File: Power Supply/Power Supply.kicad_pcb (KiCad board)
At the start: 2 copper layers, 127 x 101.6 mm, 37 parts, among them J1 Conn_01x01_Female, J2 Conn_01x01_Female, J3 Conn_01x01_Female, J4 -V_Conn, J5 +V_Conn, J6 GND_Conn, U1 LM337_TO220, U2 LM317_3PinPackage

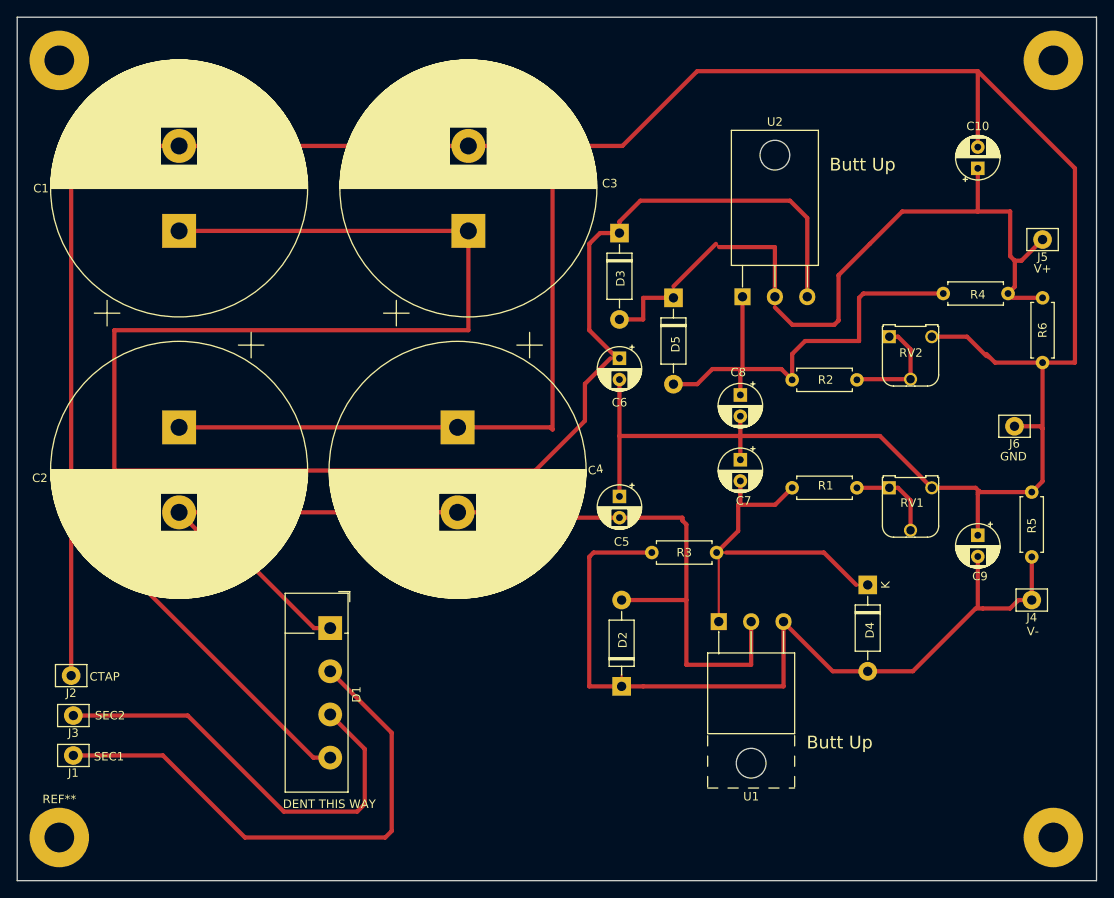
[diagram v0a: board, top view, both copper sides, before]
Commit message: ooh some new pcbs yayy
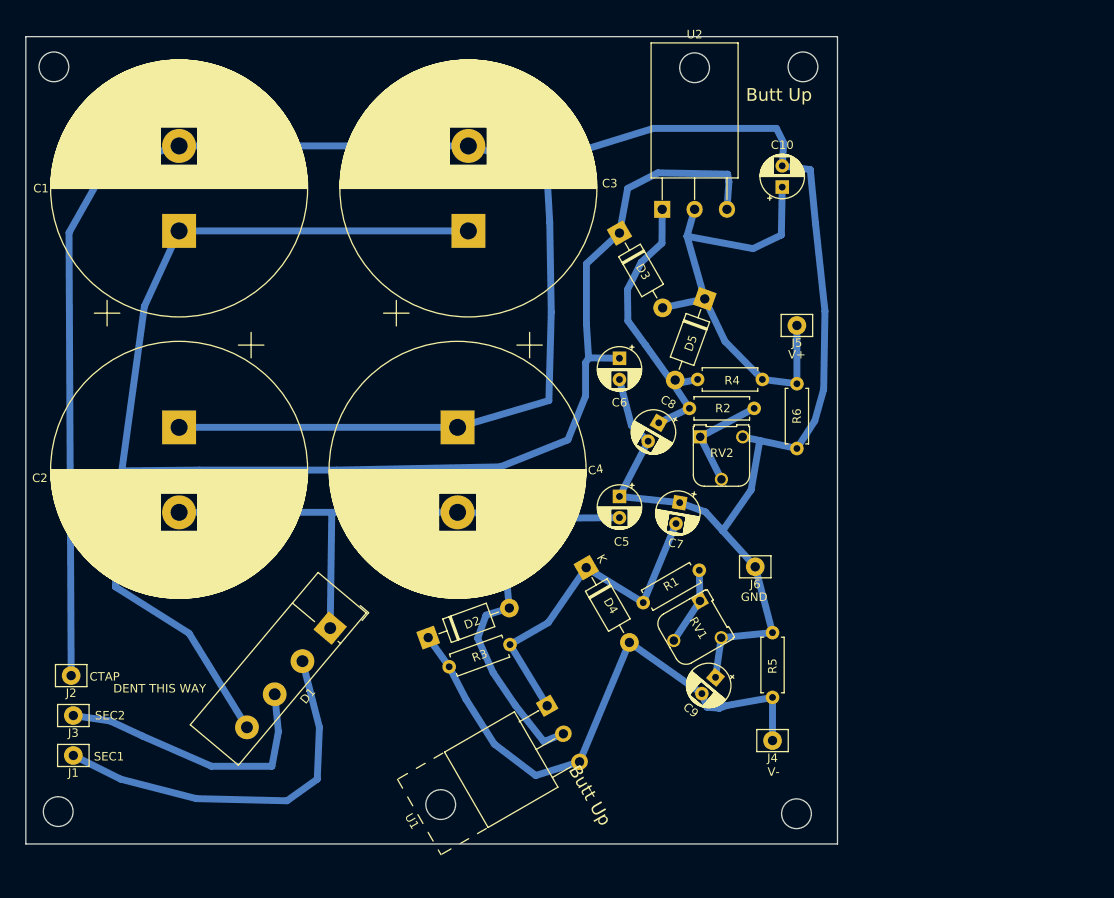
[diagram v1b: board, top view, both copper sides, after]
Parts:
- removed the REF** at (134.6, 17.8)
- removed the REF** at (134.6, 109.2)
- removed the REF** at (17.7, 109.2)
- removed the REF** at (17.7, 17.8)
- added REF**: MountingHole_3.5mm, MountingHole:MountingHole_3.5mm, F.Cu at (17.0, 18.5)
- added REF**: MountingHole_3.5mm, MountingHole:MountingHole_3.5mm, F.Cu at (17.5, 106.2)
- added REF**: MountingHole_3.5mm, MountingHole:MountingHole_3.5mm, F.Cu at (104.4, 106.4)
- added REF**: MountingHole_3.5mm, MountingHole:MountingHole_3.5mm, F.Cu at (105.2, 18.5)
- moved C9 35.1 mm to (94.9, 90.4), turned to 230 degrees
- moved J4 34.7 mm to (101.6, 97.8)
- moved J6 34.7 mm to (99.5, 77.4)
- moved R5 34.7 mm to (101.6, 92.7)
- moved D4 33.2 mm to (79.7, 77.5), turned to 300 degrees
- moved R4 30.6 mm to (100.4, 55.3)
- moved J5 30.6 mm to (104.4, 49.0)
- moved R6 30.6 mm to (104.4, 55.8)
- moved R3 27.4 mm to (63.5, 89.1), turned to 20 degrees
- moved RV1 25.9 mm to (93.0, 81.4), turned to 300 degrees
- moved RV2 25.2 mm to (93.1, 62.1)
- moved U1 23.6 mm to (75.7, 94.8), turned to 300 degrees
- moved D2 23.5 mm to (61.1, 85.7), turned to 20 degrees
- moved C10 23.1 mm to (102.7, 32.7)
- moved R1 22.1 mm to (86.4, 81.6), turned to 30 degrees
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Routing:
- net Earth: track 412.0 -> 327.1 mm
- net Net-(C1-Pad1): track 271.2 -> 205.5 mm
- net Net-(C10-Pad1): track 93.5 -> 56.7 mm
- net /VNEG: track 101.4 -> 66.6 mm
- net Net-(C2-Pad2): track 120.8 -> 99.4 mm
- net Net-(C8-Pad1): track 54.0 -> 34.1 mm
- net /SEC1: track 63.6 -> 44.6 mm
- net Net-(D1-Pad3): track 51.6 -> 33.1 mm
- net Net-(C7-Pad2): track 45.5 -> 39.4 mm
- net Net-(R1-Pad2): track 10.4 -> 9.20 mm
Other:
- board size 127 x 101.6 mm -> 95.5 x 95 mm

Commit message: uwu
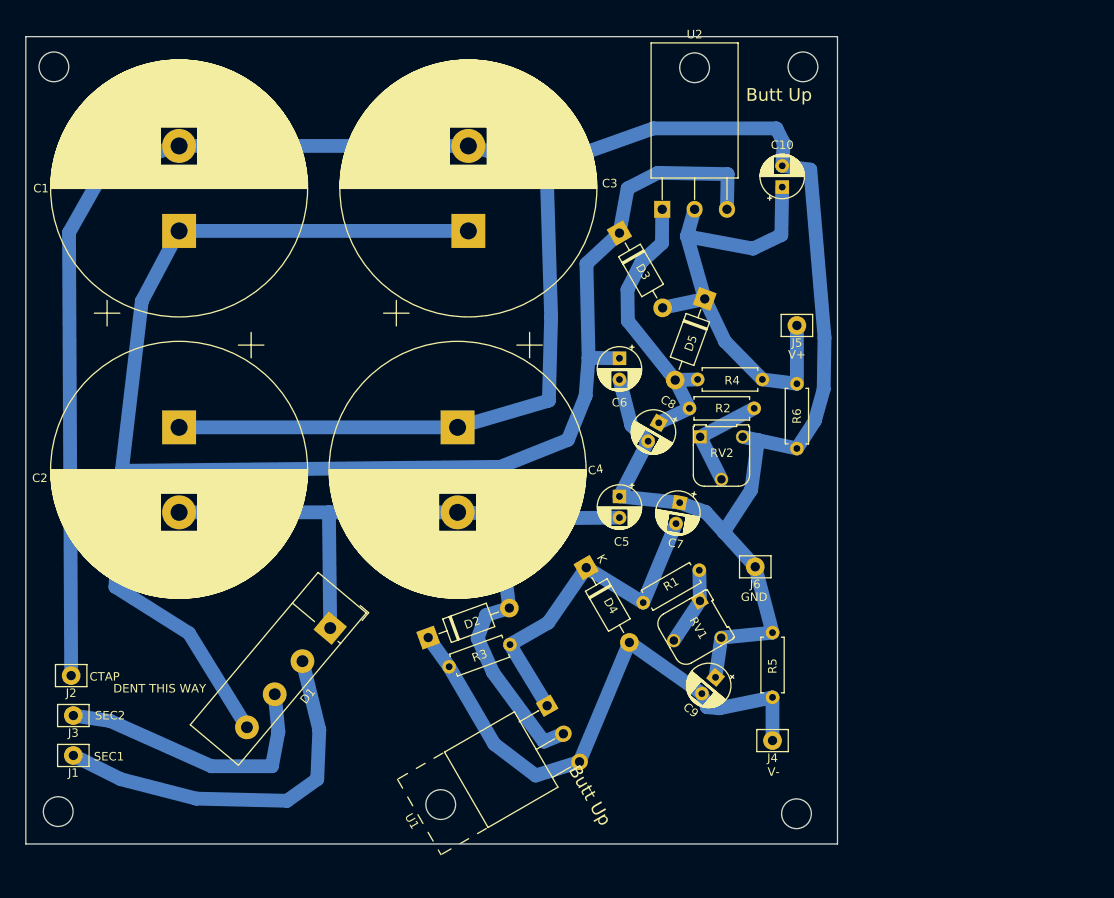
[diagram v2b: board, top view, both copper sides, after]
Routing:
- net Earth: track 327.1 -> 377.0 mm
- net Net-(C2-Pad2): track 99.4 -> 145.8 mm
- net Net-(C8-Pad1): track 34.1 -> 49.3 mm
